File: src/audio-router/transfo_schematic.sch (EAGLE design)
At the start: 15 parts

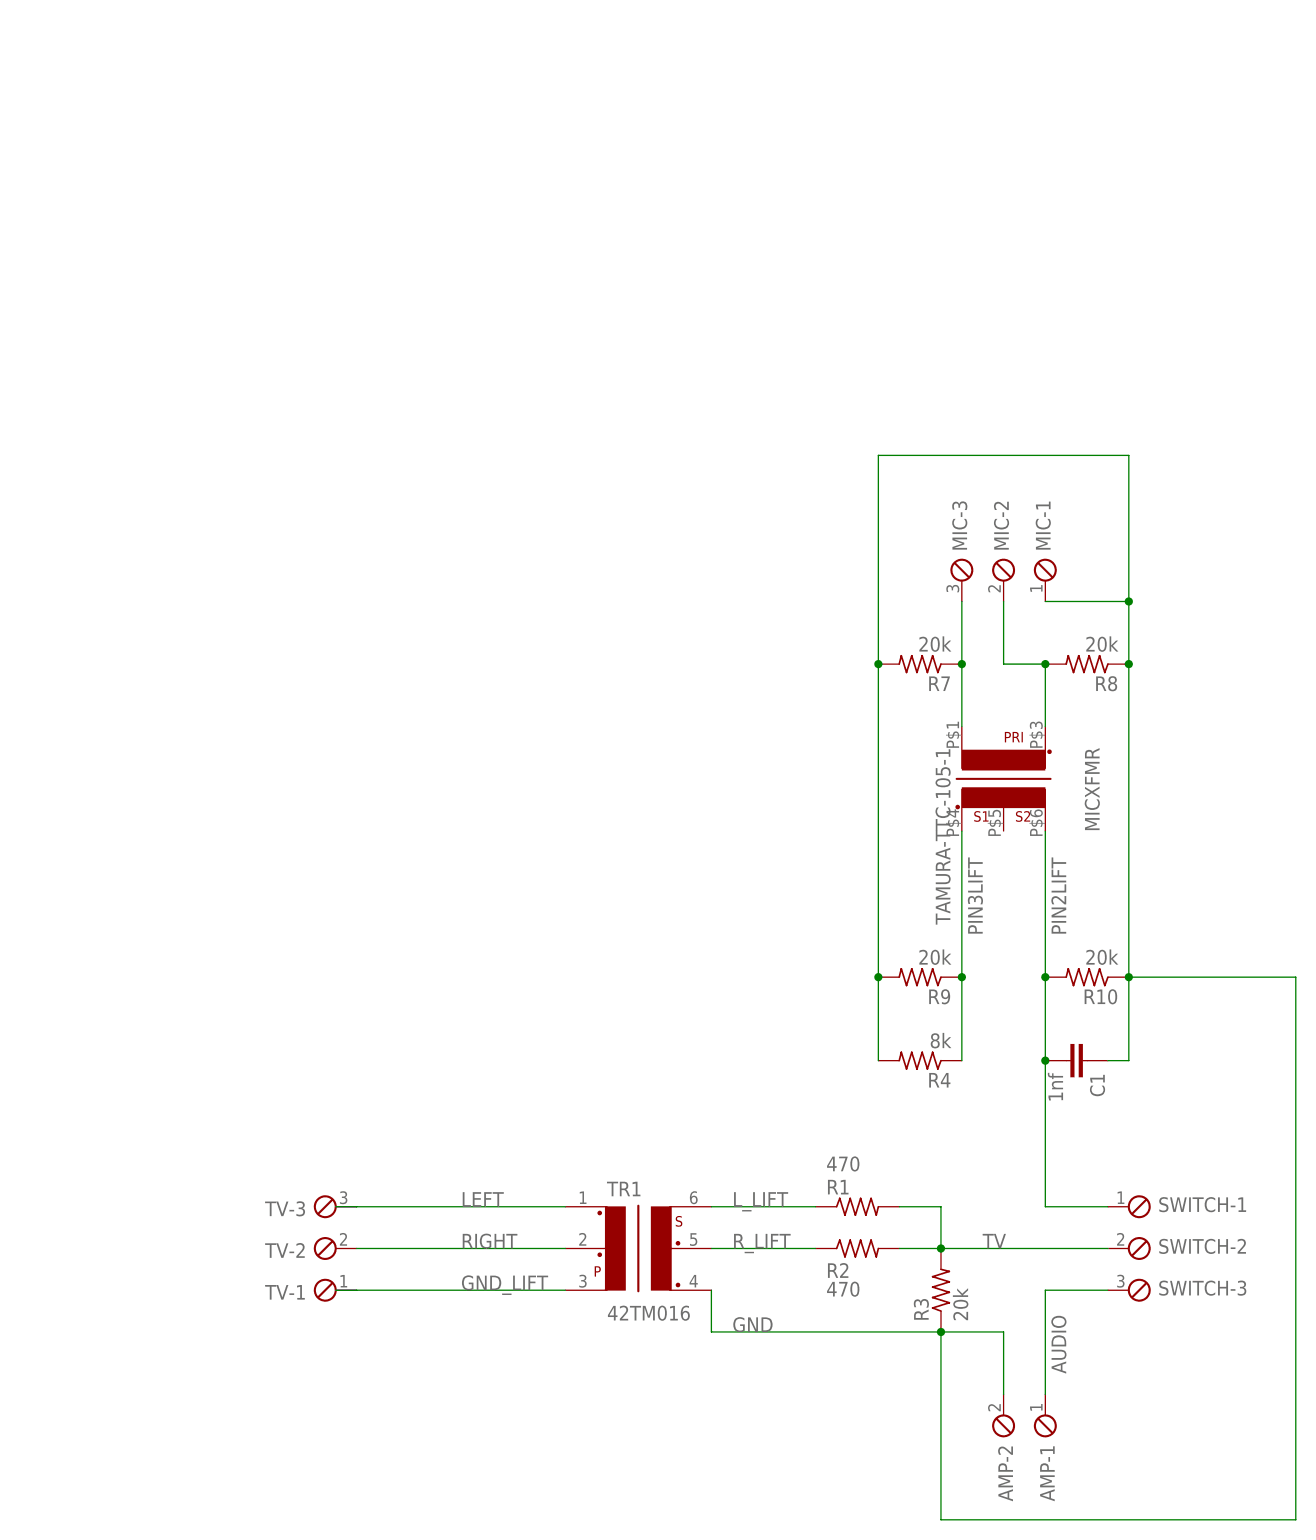
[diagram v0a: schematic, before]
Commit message: v4.3 board design
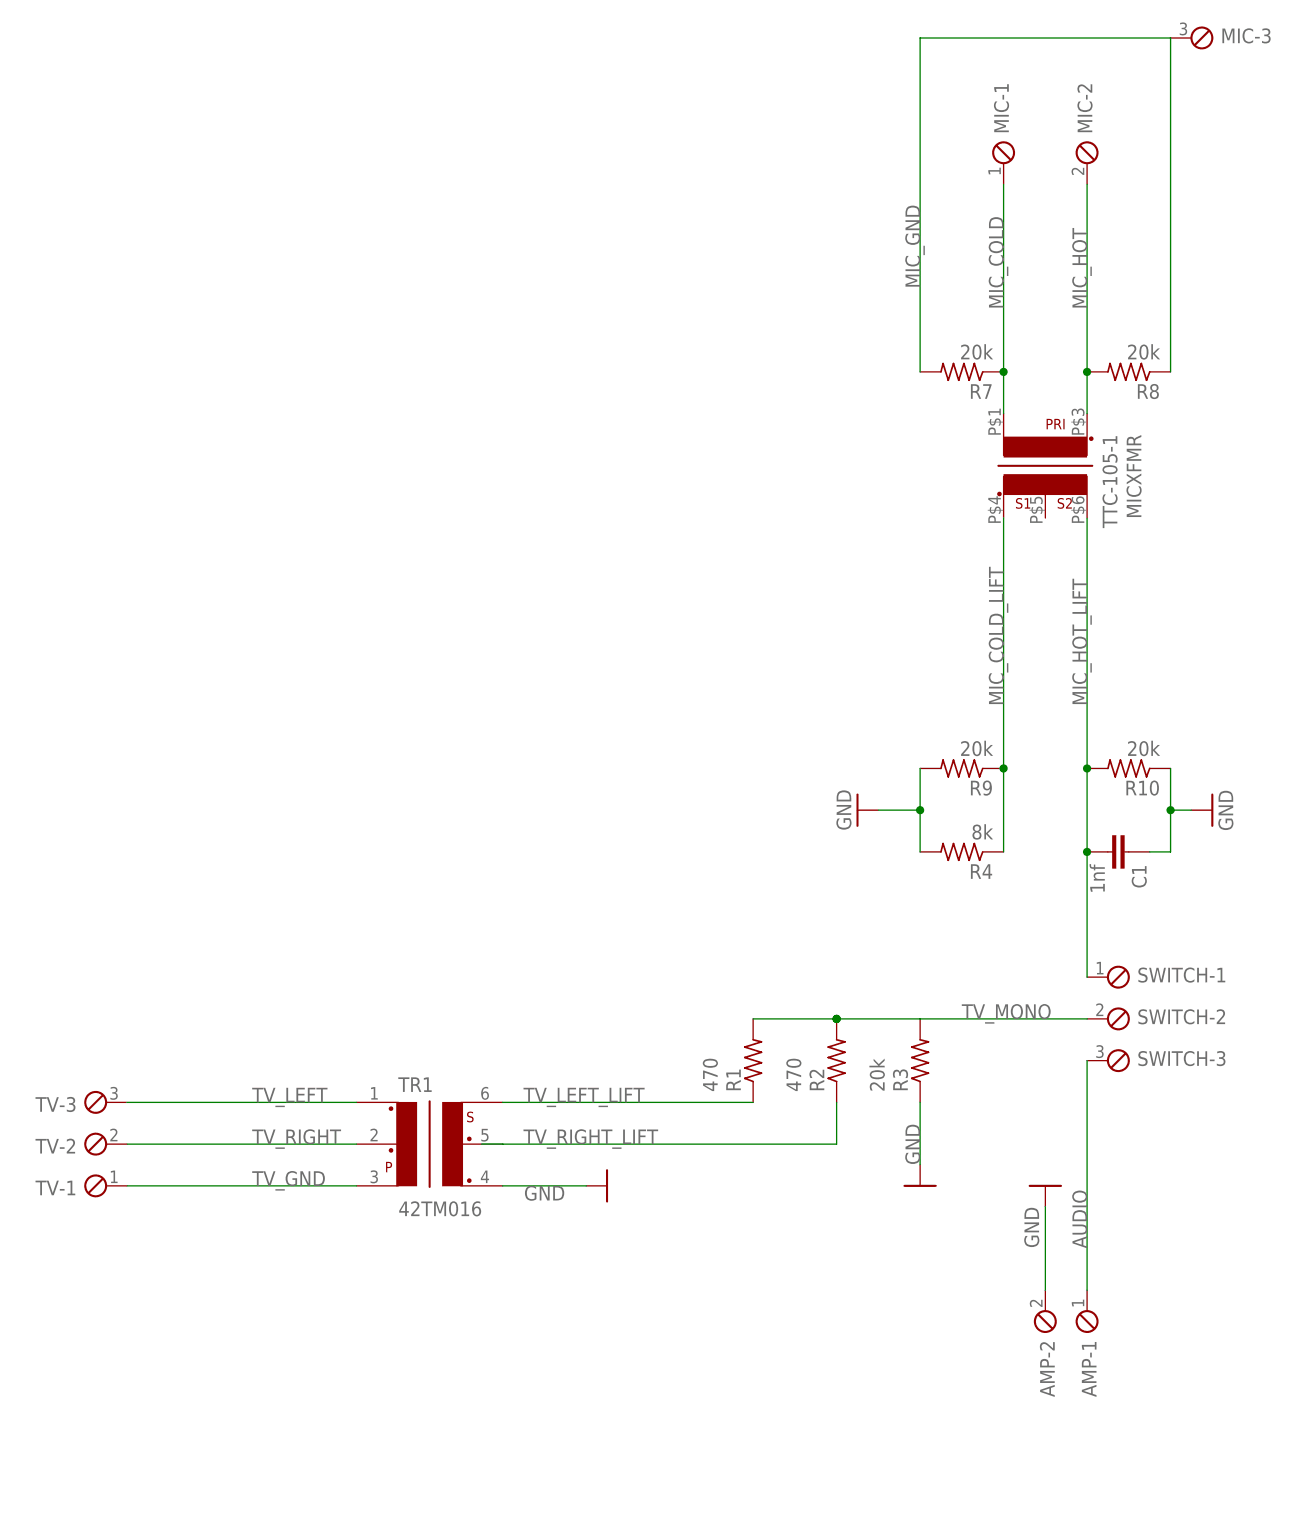
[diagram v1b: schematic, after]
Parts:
- AMP: value (none) -> TB3POL; device con-phoenix-254:MPT2 -> con-phoenix-381:MKDS1/2-3,81
- MIC, SWITCH, TV: value (none) -> TB3POL; device con-phoenix-254:MPT3 -> con-phoenix-381:MKDS1/3-3,81
- MICXFMR: value TAMURA-TTC-105-1 -> TTC-105-1
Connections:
- net GND_LIFT renamed TV_GND
- net LEFT renamed TV_LEFT
- net L_LIFT renamed TV_LEFT_LIFT
- net N$1 renamed MIC_HOT
- net PIN2LIFT renamed MIC_HOT_LIFT
- net PIN3LIFT renamed MIC_COLD_LIFT
- net RIGHT renamed TV_RIGHT
- net R_LIFT renamed TV_RIGHT_LIFT
- net TV renamed TV_MONO
- removed net N$2: MIC-3.1, MICXFMR.1, R7.1
- new net MIC_COLD: MIC-1.1, MICXFMR.1, R7.1
- new net MIC_GND: MIC-3.1, R7.2, R8.1
- net GND: no longer MIC-1.1, R7.2, R8.1
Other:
- moved on the sheet: AMP-1, AMP-2, C1, MIC-1, MIC-2, MIC-3, MICXFMR, R1, R10, R2, R3, R4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
